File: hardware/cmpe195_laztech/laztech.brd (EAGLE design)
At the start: 68.6 x 61 mm, 27 parts

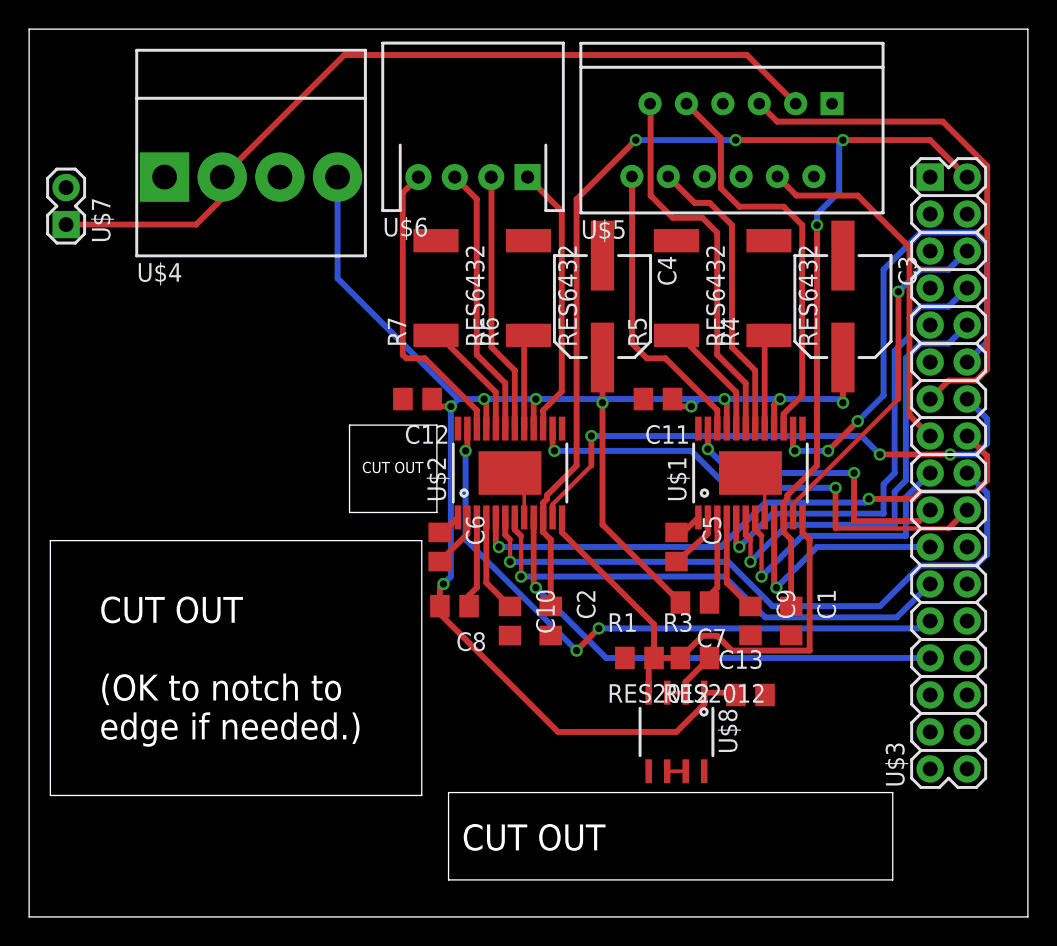
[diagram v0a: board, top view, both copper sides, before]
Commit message: Got brd and sch back on track.
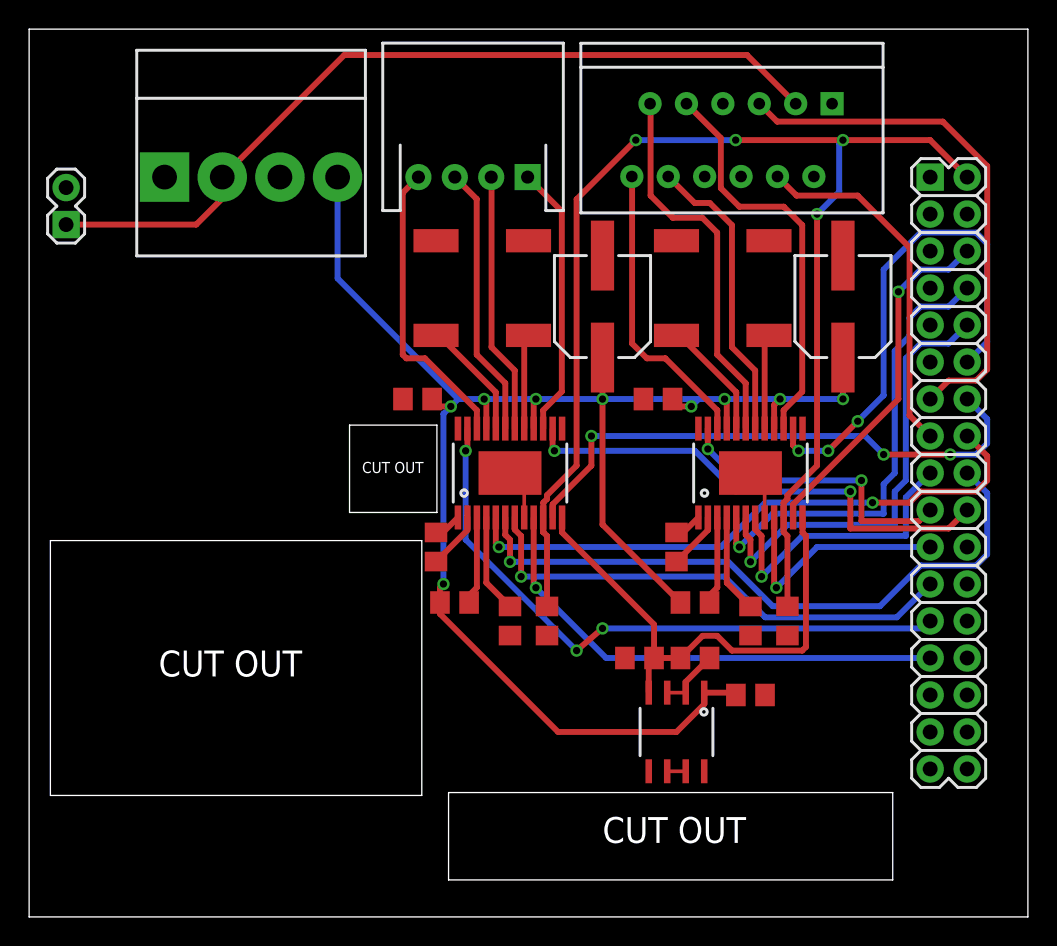
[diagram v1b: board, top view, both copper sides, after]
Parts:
- moved C8 0.25 mm to (29.2, 21.6)
- moved C1 0.25 mm to (52.1, 20.3)
- moved C2 0.25 mm to (35.6, 20.3)
- moved C6 0.25 mm to (27.9, 25.4)
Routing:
- net +24V: track 120.4 -> 119.8 mm
- net VREF: track 35.9 -> 35.4 mm
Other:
- board text removed: "CUT OUT (OK to notch to edge if needed.)"
